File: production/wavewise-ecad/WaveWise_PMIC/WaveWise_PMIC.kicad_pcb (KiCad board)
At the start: 4 copper layers, 94 x 114.3 mm, 53 parts, among them IC1 LV14360PDDAR, J1 24V output, J10 5031590200, J11 5031590200, J12 Regulated 48V Input, J2 Inverter Inputs, J3 Conn_01x03_Pin, J4 Conn_01x04_Pin, J5 5031590400, J6 5031590400, J7 5V output, J8 5031590800, J9 5031590300, K1 Relay_SPST-NO, Q2 2N2219, U1 Raspberry Pi Pico, U2 Pololu_DRV8711_Motor_Driver, U4 LM2576HVS-5.0_NOPB

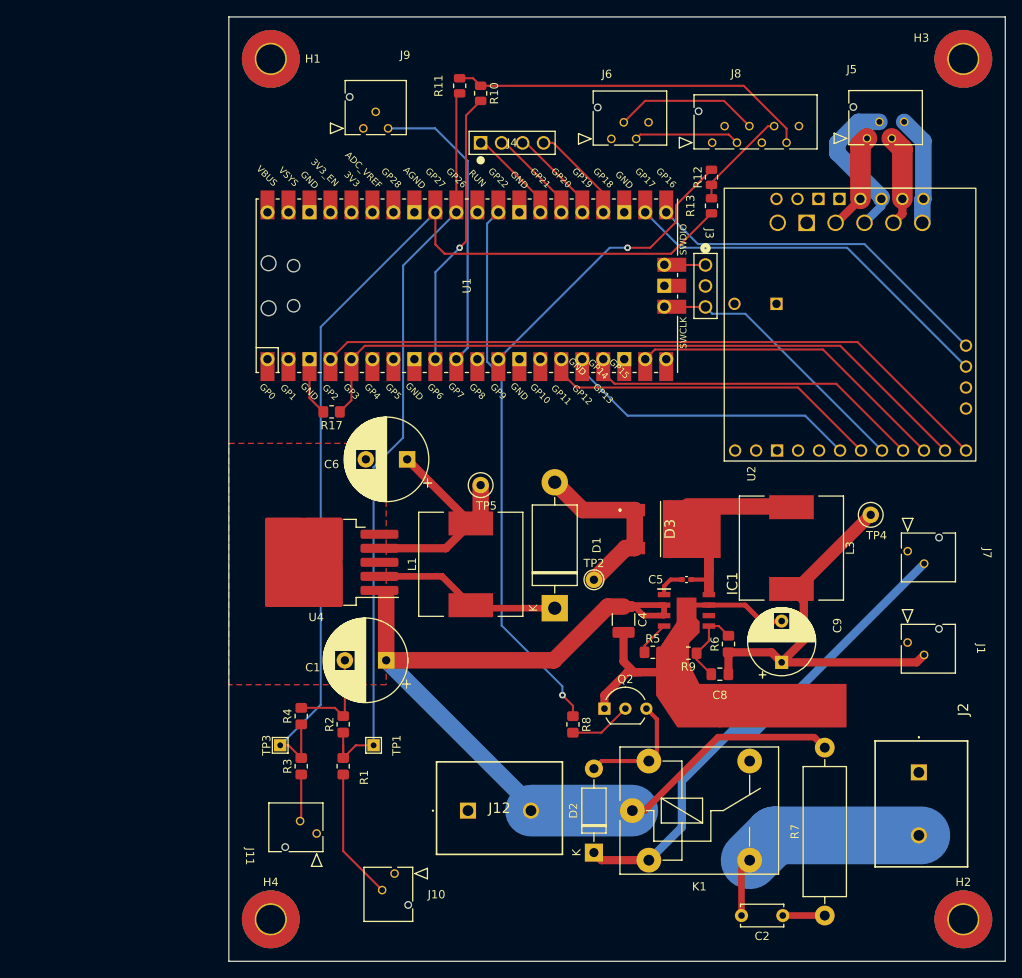
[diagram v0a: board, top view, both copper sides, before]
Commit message: Prelim board layout
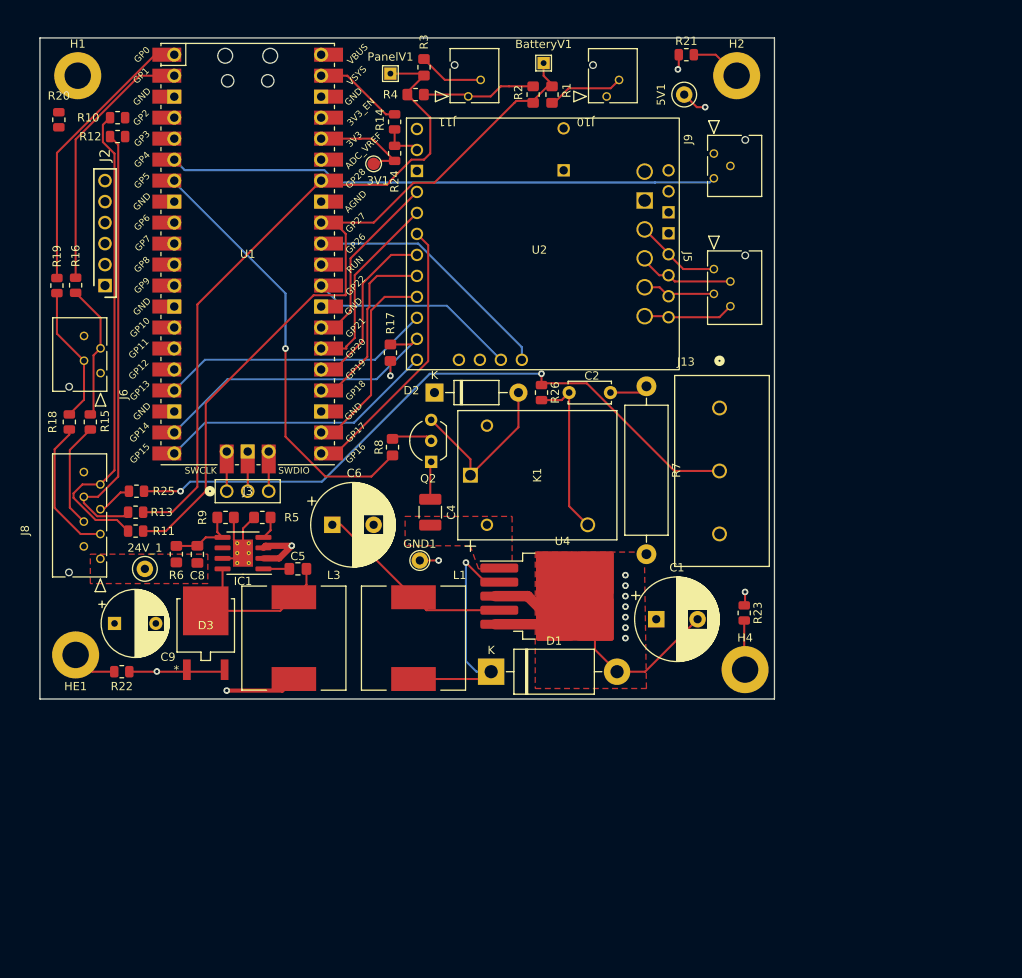
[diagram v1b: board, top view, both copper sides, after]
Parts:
- removed H3: MountingHole, MountingHole:MountingHole_3.5mm_Pad_TopBottom
- removed J1: 24V output, Unchecked:2pinmolex
- removed J12: Regulated 48V Input, Unchecked:1731721
- removed J4: Conn_01x04_Pin, Unchecked:61300411121
- removed J7: 5V output, Unchecked:2pinmolex
- removed TP1, TP3: TestPoint, TestPoint:TestPoint_THTPad_1.5x1.5mm_Drill0.7mm
- removed TP2: TestPoint, TestPoint:TestPoint_THTPad_D2.0mm_Drill1.0mm
- removed TP4: 24V TP, TestPoint:TestPoint_Loop_D1.80mm_Drill1.0mm_Beaded
- removed TP5: 5V TP, TestPoint:TestPoint_Loop_D1.80mm_Drill1.0mm_Beaded
- added 24V_1: 24V TP, TestPoint:TestPoint_Loop_D1.80mm_Drill1.0mm_Beaded, F.Cu at (63.5, 115.1)
- added 3V1: TestPoint, TestPoint:TestPoint_Pad_D1.5mm, F.Cu at (91.2, 66.0)
- added 5V1: 5V TP, TestPoint:TestPoint_Loop_D1.80mm_Drill1.0mm_Beaded, F.Cu at (128.8, 57.7)
- added BatteryV1: TestPoint, TestPoint:TestPoint_THTPad_1.5x1.5mm_Drill0.7mm, F.Cu at (111.8, 53.8)
- added GND1: TestPoint, TestPoint:TestPoint_THTPad_D2.0mm_Drill1.0mm, F.Cu at (96.8, 114.0)
- added HE1: MountingHole, MountingHole:MountingHole_3.2mm_M3_ISO7380_Pad, F.Cu at (55.1, 125.5)
- added J13: Screw_Terminal_01x03, Unchecked:CONN_1731734_PXC, F.Cu at (133.1, 95.6)
- added PanelV1: TestPoint, TestPoint:TestPoint_THTPad_1.5x1.5mm_Drill0.7mm, F.Cu at (93.2, 55.1)
- added R14: 0, Resistor_SMD:R_0805_2012Metric, F.Cu at (93.7, 61.0)
- added R15: 0, Resistor_SMD:R_0805_2012Metric, F.Cu at (56.9, 97.3)
- added R16: 0, Resistor_SMD:R_0805_2012Metric, F.Cu at (55.1, 80.7)
- added R18: 0, Resistor_SMD:R_0805_2012Metric, F.Cu at (54.4, 97.3)
- added R19: 0, Resistor_SMD:R_0805_2012Metric, F.Cu at (52.9, 80.8)
- added R20: 0, Resistor_SMD:R_0805_2012Metric, F.Cu at (53.1, 60.7)
- added R21: 0, Resistor_SMD:R_0805_2012Metric, F.Cu at (129.0, 52.8)
- added R22: 0, Resistor_SMD:R_0805_2012Metric, F.Cu at (60.7, 127.5)
- added R23: 0, Resistor_SMD:R_0805_2012Metric, F.Cu at (136.0, 120.4)
- added R24: 0, Resistor_SMD:R_0805_2012Metric, F.Cu at (93.7, 64.8)
- added R25: 0, Resistor_SMD:R_0805_2012Metric, F.Cu at (62.5, 105.7)
- added R26: 0, Resistor_SMD:R_0805_2012Metric, F.Cu at (111.5, 93.7)
- C5: footprint Capacitor_SMD:C_0402_1005Metric_Pad0.74x0.62mm_HandSolder -> Capacitor_SMD:C_0805_2012Metric_Pad1.18x1.45mm_HandSolder
- D3: footprint SBR10200CTL-13:ZLDO1117K50TC -> Unchecked:TO-252DPAK_DIO
- H1, H2, H4: footprint MountingHole:MountingHole_3.5mm_Pad_TopBottom -> MountingHole:MountingHole_3.2mm_M3_ISO7380_Pad
- IC1: footprint LV14360PDDAR:SOIC127P600X170-9N -> Package_SO:SOIC-8-1EP_3.9x4.9mm_P1.27mm_EP2.41x3.3mm_ThermalVias
- J2: value Inverter Inputs -> Conn_01x06_Pin; footprint Unchecked:1731721 -> Unchecked:61300611121
- J5, J6: footprint Footprints:4pinmolex -> Unchecked:4pinmolex
- J8: footprint Footprints:8pinmolex -> Unchecked:8pinmolex
- K1: value Relay_SPST-NO -> AWHSH105D00G; footprint Relay_THT:Relay_SPDT_Finder_36.11 -> Unchecked:AWHSH105D00G
- U4: footprint Package_TO_SOT_SMD:TO-263-5_TabPin3 -> Package_TO_SOT_SMD:TO-263-5_TabPin6
- moved J2 114.8 mm to (58.7, 80.8), turned to 90 degrees
- moved H2 105.7 mm to (135.1, 55.4)
- moved J10 97.5 mm to (119.4, 57.9), turned to 0 degrees
- moved J11 91.1 mm to (102.6, 57.9), turned to 0 degrees
- moved J8 89.6 mm to (58.1, 113.8), turned to 90 degrees
- moved R3 85.9 mm to (97.3, 54.4), turned to -90 degrees
- moved R1 85.1 mm to (112.8, 57.7)
- moved C9 80.9 mm to (59.8, 121.7), turned to 0 degrees
- moved R2 79.6 mm to (110.5, 57.7)
- moved R13 79.0 mm to (62.4, 108.2), turned to 0 degrees
- moved R4 76.5 mm to (96.3, 57.7), turned to 0 degrees
- moved R12 72.1 mm to (60.2, 62.7), turned to 0 degrees
- moved J6 68.0 mm to (58.1, 91.4), turned to 90 degrees
- moved R6 67.7 mm to (67.3, 113.3)
- moved R7 67.6 mm to (124.2, 93.0), turned to -90 degrees
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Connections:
- net /Connectors/AOUT1 renamed /AOUT1
- net /Connectors/AOUT2 renamed /AOUT2
- net /Connectors/BOUT1 renamed /BOUT1
- net /Connectors/BOUT2 renamed /BOUT2
- C2 pad 2: /Connectors/Inverter_Input -> /Inverter_Input
- H1 pad 1: (no net) -> Net-(H1-Pad1)
- H2 pad 1: (no net) -> Net-(H2-Pad1)
- H4 pad 1: (no net) -> Net-(H4-Pad1)
- J2 pad 1: GND -> /Connectors/GPIO4
- J2 pad 2: /Connectors/Inverter_Input -> /Connectors/GPIO3
- J3 pad 1: /Connectors/DIO -> /Connectors/SWCLK
- J3 pad 3: /CLK -> /Connectors/SWDIO
- J6 pad 2: /Connectors/rockblock_RX -> /Connectors/rockblock_TX
- J6 pad 3: /Connectors/rockblock_TX -> /Connectors/rockblock_RX
- J8 pad 3: /Connectors/rockblock_TX -> /Connectors/SICO_TX
- J8 pad 4: /Connectors/rockblock_RX -> /Connectors/SICO_RX
- R1 pad 2: /BATT_SENS -> /Connectors/Batt V Sense
- R10 pad 2: /DIO_BatterySense -> /Connectors/BATT_SENSE_DIO
- R11 pad 2: /BATT_SENS -> /Connectors/Batt V Sense
- R12 pad 2: /panel_sense_DIO -> /Connectors/PANEL_SENSE_DIO
- R13 pad 2: /Panel_Sense -> /Connectors/Panel V Sense
- R17 pad 1: /MOTOR_RESET -> /PICO (BICO)/MOTOR_RESET
- R2 pad 1: /BATT_SENS -> /Connectors/Batt V Sense
- R3 pad 2: /Panel_Sense -> /Connectors/Panel V Sense
- R4 pad 1: /Panel_Sense -> /Connectors/Panel V Sense
- R8 pad 1: /PUMP_CTL -> /PICO (BICO)/PUMP_CTRL
- U1 pad 1: /PICO (BICO)/B_TX -> /Connectors/BICO_UART_TX
- U1 pad 10: /Connectors/PWM_Servo -> /Connectors/GPIO2
- U1 pad 11: unconnected-(U1-GPIO8-Pad11) -> /Connectors/GPIO3
- U1 pad 12: /panel_sense_DIO -> /Connectors/GPIO4
- U1 pad 14: /PICO (BICO)/SCK -> unconnected-(U1-GPIO10-Pad14)
- U1 pad 15: /PICO (BICO)/MOSI1 -> unconnected-(U1-GPIO11-Pad15)
- U1 pad 16: /PICO (BICO)/MISO1 -> unconnected-(U1-GPIO12-Pad16)
- U1 pad 17: /PICO (BICO)/SCS -> /PICO (BICO)/MOTOR_SLP
- U1 pad 19: /~SLP -> /PICO (BICO)/MOTOR_RESET
- U1 pad 2: /PICO (BICO)/B_RX -> /Connectors/BICO_UART_RX
- U1 pad 20: unconnected-(U1-GPIO15-Pad20) -> /PICO (BICO)/MOTOR_FLT
- U1 pad 21: /BEMF -> /PICO (BICO)/MOTOR_SPI0_RX
- U1 pad 22: /STALL -> /PICO (BICO)/MOTOR_SPI0_CSn
- U1 pad 24: /GPIO1 -> /PICO (BICO)/MOTOR_SPI0_SCK
- U1 pad 25: /GPIO2 -> /PICO (BICO)/MOTOR_SPI0_TX
- U1 pad 26: /GPIO3 -> /PICO (BICO)/MOTOR_DIR/AIN2
- U1 pad 27: /GPIO4 -> /PICO (BICO)/MOTOR_STEP/AIN1
- U1 pad 29: /PUMP_CTL -> /PICO (BICO)/MOTOR_STALL
- U1 pad 31: /BATT_SENS -> /PICO (BICO)/MOTOR_BEMF
- U1 pad 32: /Panel_Sense -> /Connectors/Batt V Sense
- U1 pad 33: unconnected-(U1-AGND-Pad33) -> GND
- U1 pad 34: unconnected-(U1-GPIO28_ADC2-Pad34) -> /Connectors/Panel V Sense
- U1 pad 36: unconnected-(U1-3V3-Pad36) -> +3.3V
- U1 pad 4: /MOTOR_FLT -> /Connectors/BATT_SENSE_DIO
- U1 pad 41: /CLK -> /Connectors/SWCLK
- U1 pad 43: /Connectors/DIO -> /Connectors/SWDIO
- U1 pad 5: /MOTOR_RESET -> /Connectors/PANEL_SENSE_DIO
- U1 pad 6: unconnected-(U1-GPIO4-Pad6) -> /Connectors/PWM_Servo
- U1 pad 7: unconnected-(U1-GPIO5-Pad7) -> /PICO (BICO)/PUMP_CTRL
- U1 pad 9: /DIO_BatterySense -> /Connectors/GPIO1
- U2 pad 10: /MOTOR_FLT -> /PICO (BICO)/MOTOR_FLT
- U2 pad 11: /MOTOR_RESET -> /PICO (BICO)/MOTOR_RESET
- U2 pad 12: /~SLP -> /PICO (BICO)/MOTOR_SLP
- U2 pad 13: /PICO (BICO)/SCS -> /PICO (BICO)/MOTOR_SPI0_CSn
- U2 pad 14: /CLK -> /PICO (BICO)/MOTOR_SPI0_SCK
- U2 pad 15: /PICO (BICO)/MOSI1 -> /PICO (BICO)/MOTOR_SPI0_TX
- U2 pad 16: /PICO (BICO)/MISO1 -> /PICO (BICO)/MOTOR_SPI0_RX
- U2 pad 17: unconnected-(U2-DIR-Pad17) -> /PICO (BICO)/MOTOR_DIR/AIN2
- U2 pad 18: unconnected-(U2-STEP-Pad18) -> /PICO (BICO)/MOTOR_STEP/AIN1
- U2 pad 19: unconnected-(U2-ICREF-Pad19) -> /Pneumatic Control/ICREF
- U2 pad 6: /BEMF -> /PICO (BICO)/MOTOR_BEMF
- U2 pad 7: /STALL -> /PICO (BICO)/MOTOR_STALL
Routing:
- net /Panel_Sense: track 119.3 -> 0.00 mm
- net +48V: track 116.6 -> 7.59 mm, vias 0 -> 1
- net +24V: track 117.5 -> 8.71 mm, vias 0 -> 1
- net +5V: track 143.8 -> 38.5 mm, vias 0 -> 1
- net /Connectors/Batt V Sense: track 0.00 -> 92.2 mm
- net /BATT_SENS: track 92.1 -> 0.00 mm
- net /MOTOR_RESET: track 84.7 -> 0.00 mm
- net /MOTOR_FLT: track 83.2 -> 0.00 mm
- net /Connectors/Panel V Sense: track 0.00 -> 81.7 mm
- net Net-(J13-Pin_2): track 0.00 -> 81.4 mm, vias 0 -> 2
- net /PUMP_CTL: track 65.9 -> 0.00 mm, vias 1 -> 0
- net /PICO (BICO)/PUMP_CTRL: track 0.00 -> 52.8 mm, vias 0 -> 1
- net /Connectors/Inverter_Input: track 50.9 -> 0.00 mm
- net /STALL: track 46.6 -> 0.00 mm
- net /BEMF: track 43.0 -> 0.00 mm
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- added copper zone on F.Cu, net +24V
- added copper zone on In1.Cu, net +24V
- added copper zone on F.Cu, net +48V
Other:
- board size 94 x 114.3 mm -> 88.9 x 80 mm
